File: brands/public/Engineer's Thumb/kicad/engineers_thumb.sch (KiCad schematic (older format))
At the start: 46 parts, among them CN1 IN, CN2 OUT, IC1 TL072, IC2 TL072, IC3 CA3080, P1 1M Lin, P2 1M Lin, P3 1M Log, P4 1M Lin, P5 10k Log, Q1 BC327, SW1 SW_3PDT, SW2 SW_ON-OFF_SINGLE

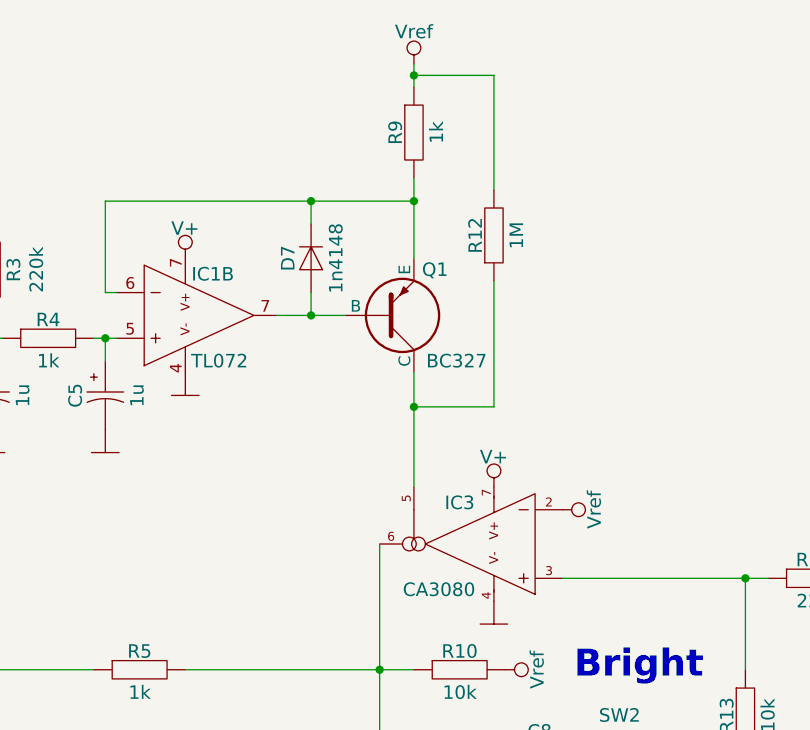
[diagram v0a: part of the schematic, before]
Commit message: Engineer's Thumb
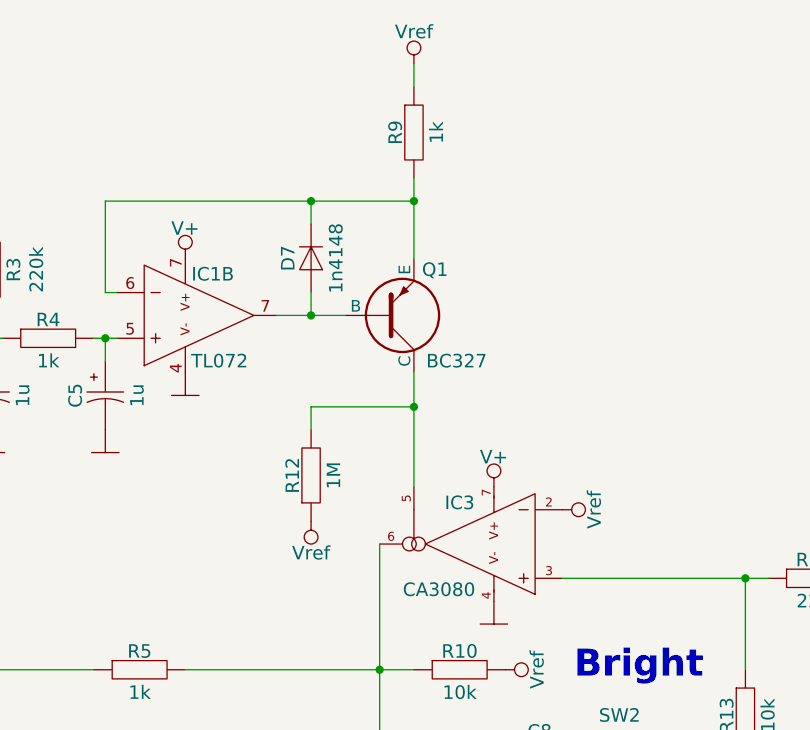
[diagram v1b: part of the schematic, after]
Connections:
- net at IC3.5, Q1.1 (C): now also R12.2; no longer R12.1
- net at R9.1: no longer R12.2
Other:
- moved on the sheet: R12
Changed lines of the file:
@@
 L RESISTOR R12
 U 1 1 544F9523
-P 7250 1500
-F 0 "R12" H 7250 1580 59  0000 C CNN
-F 1 "1M" H 7250 1400 59  0000 C CNN
-F 2 "drow:resistor_7.5mm" H 7100 1540 60  0001 C CNN
-F 3 "" H 7100 1540 60  0000 C CNN
-	1    7250 1500
+P 6450 2550
+F 0 "R12" H 6450 2630 59  0000 C CNN
+F 1 "1M" H 6450 2450 59  0000 C CNN
+F 2 "drow:resistor_7.5mm" H 6300 2590 60  0001 C CNN
+F 3 "" H 6300 2590 60  0000 C CNN
+	1    6450 2550
 	0    -1   -1   0
 $EndComp
@@
 	6450 1450 6450 1350
 Wire Wire Line
-	7250 2250 6900 2250
-Wire Wire Line
 	6900 2100 6900 2600
 Wire Wire Line
@@
 	1    0    0    -1
 $EndComp
-Connection ~ 6900 800
 Wire Wire Line
 	6900 750  6900 850
-Wire Wire Line
-	7250 800  6900 800
-Wire Wire Line
-	7250 1300 7250 800
-Wire Wire Line
-	7250 1700 7250 2250
 Wire Wire Line
 	6900 1250 6900 1600
@@
 Wire Wire Line
 	4800 5250 4800 5350
+Wire Wire Line
+	6900 2250 6450 2250
+Wire Wire Line
+	6450 2250 6450 2350
+$Comp
+L Vref #PWR?
+U 1 1 54B3E7A5
+P 6450 2750
+F 0 "#PWR?" H 6450 2720 20  0001 C CNN
+F 1 "Vref" H 6450 2890 59  0000 C CNN
+F 2 "" H 6450 2750 60  0000 C CNN
+F 3 "" H 6450 2750 60  0000 C CNN
+	1    6450 2750
+	-1   0    0    1
+$EndComp
 $EndSCHEMATC
